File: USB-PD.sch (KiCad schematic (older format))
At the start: 54 parts, among them IC3 TPS7A0518PDBVT, J1 1053131102, J11 E8124-015-01, Q10 Si7223DN, Q11 Si7223DN, Q9 SQS401EN-T1_BE3, U12 STUSB4500QTR, U14 LTC4418IUF#PBF

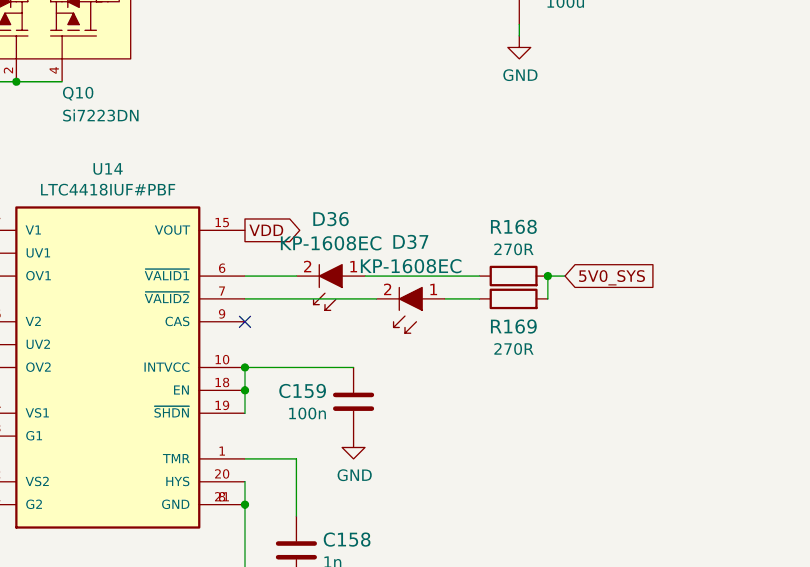
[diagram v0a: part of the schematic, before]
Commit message: All routes connected
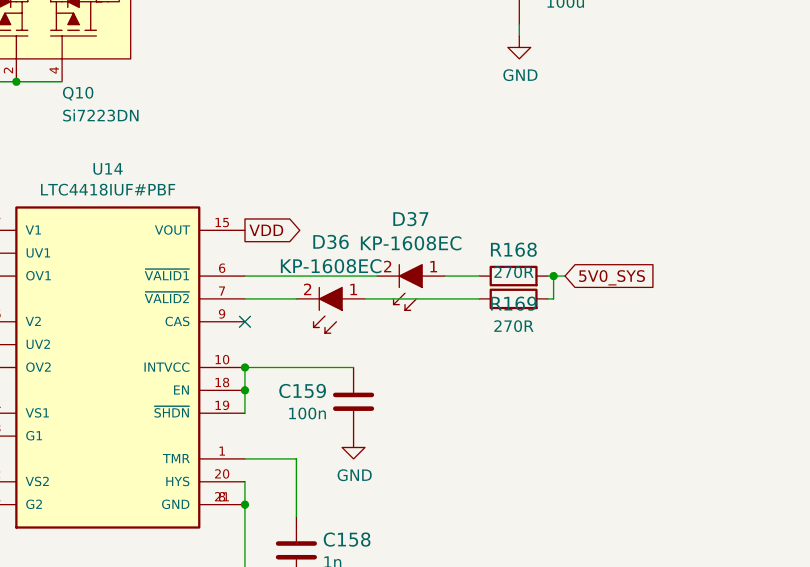
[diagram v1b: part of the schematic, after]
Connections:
- net at U14.6 (~VALID1): now also D37.2; no longer D36.2
- net at U14.7 (~VALID2): now also D36.2; no longer D37.2
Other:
- moved on the sheet: D36, D37, R168, R169
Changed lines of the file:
@@
 L sc606-baseboard:KP-1608EC D?
 U 1 1 62106E33
-P 9650 8200
+P 9650 8300
 AR Path="/61D43102/62106E33" Ref="D?"  Part="1"
 AR Path="/61D49FDE/62106E33" Ref="D?"  Part="1"
 AR Path="/623AED4D/62106E33" Ref="D36"  Part="1"
-F 0 "D36" H 9600 7953 60  0000 C CNN
-F 1 "KP-1608EC" H 9600 8059 60  0000 C CNN
-F 2 "sc606-baseboard-footprints:LED_0603" H 9850 8400 60  0001 L CNN
-F 3 "https://www.farnell.com/datasheets/1854072.pdf" H 9850 8500 60  0001 L CNN
-F 4 "KP-1608EC" H 9850 8700 60  0001 L CNN "MPN"
-F 5 "KINGBRIGHT" H 9860 8820 60  0001 L CNN "Manufacturer"
-	1    9650 8200
+F 0 "D36" H 9600 8053 60  0000 C CNN
+F 1 "KP-1608EC" H 9600 8159 60  0000 C CNN
+F 2 "sc606-baseboard-footprints:LED_0603" H 9850 8500 60  0001 L CNN
+F 3 "https://www.farnell.com/datasheets/1854072.pdf" H 9850 8600 60  0001 L CNN
+F 4 "KP-1608EC" H 9850 8800 60  0001 L CNN "MPN"
+F 5 "KINGBRIGHT" H 9860 8920 60  0001 L CNN "Manufacturer"
+	1    9650 8300
 	-1   0    0    1
 $EndComp
@@
 L sc606-baseboard:KP-1608EC D?
 U 1 1 6211676C
-P 10000 8300
+P 10000 8200
 AR Path="/61D43102/6211676C" Ref="D?"  Part="1"
 AR Path="/61D49FDE/6211676C" Ref="D?"  Part="1"
 AR Path="/623AED4D/6211676C" Ref="D37"  Part="1"
-F 0 "D37" H 9950 8053 60  0000 C CNN
-F 1 "KP-1608EC" H 9950 8159 60  0000 C CNN
-F 2 "sc606-baseboard-footprints:LED_0603" H 10200 8500 60  0001 L CNN
-F 3 "https://www.farnell.com/datasheets/1854072.pdf" H 10200 8600 60  0001 L CNN
-F 4 "KP-1608EC" H 10200 8800 60  0001 L CNN "MPN"
-F 5 "KINGBRIGHT" H 10210 8920 60  0001 L CNN "Manufacturer"
-	1    10000 8300
+F 0 "D37" H 9950 7953 60  0000 C CNN
+F 1 "KP-1608EC" H 9950 8059 60  0000 C CNN
+F 2 "sc606-baseboard-footprints:LED_0603" H 10200 8400 60  0001 L CNN
+F 3 "https://www.farnell.com/datasheets/1854072.pdf" H 10200 8500 60  0001 L CNN
+F 4 "KP-1608EC" H 10200 8700 60  0001 L CNN "MPN"
+F 5 "KINGBRIGHT" H 10210 8820 60  0001 L CNN "Manufacturer"
+	1    10000 8200
 	-1   0    0    1
 $EndComp
@@
 L sc606-baseboard:R_270R_0603 R168
 U 1 1 6201E54F
+P 10500 8300
+F 0 "R168" H 10500 8513 60  0000 C CNN
+F 1 "R_270R_0603" H 10500 8150 60  0001 C CNN
+F 2 "sc606-baseboard-footprints:0603-res" H 10700 8500 60  0001 L CNN
+F 3 "https://industrial.panasonic.com/cdbs/www-data/pdf/RDA0000/AOA0000C304.pdf" H 10500 8300 50  0001 C CNN
+F 4 "Panasonic" H 10700 8700 60  0001 L CNN "Manufacturer"
+F 5 "ERJ3EKF2700V" H 10700 8600 60  0001 L CNN "MPN"
+F 6 "270R" H 10500 8415 50  0000 C CNN "Val"
+	1    10500 8300
+	1    0    0    -1
+$EndComp
+$Comp
+L sc606-baseboard:R_270R_0603 R169
+U 1 1 6201EDA2
 P 10500 8200
-F 0 "R168" H 10500 8413 60  0000 C CNN
+F 0 "R169" H 10500 8077 60  0000 C CNN
 F 1 "R_270R_0603" H 10500 8050 60  0001 C CNN
 F 2 "sc606-baseboard-footprints:0603-res" H 10700 8400 60  0001 L CNN
@@
 F 4 "Panasonic" H 10700 8600 60  0001 L CNN "Manufacturer"
 F 5 "ERJ3EKF2700V" H 10700 8500 60  0001 L CNN "MPN"
-F 6 "270R" H 10500 8315 50  0000 C CNN "Val"
+F 6 "270R" H 10500 7979 50  0000 C CNN "Val"
 	1    10500 8200
 	1    0    0    -1
 $EndComp
-$Comp
-L sc606-baseboard:R_270R_0603 R169
-U 1 1 6201EDA2
-P 10500 8300
-F 0 "R169" H 10500 8177 60  0000 C CNN
-F 1 "R_270R_0603" H 10500 8150 60  0001 C CNN
-F 2 "sc606-baseboard-footprints:0603-res" H 10700 8500 60  0001 L CNN
-F 3 "https://industrial.panasonic.com/cdbs/www-data/pdf/RDA0000/AOA0000C304.pdf" H 10500 8300 50  0001 C CNN
-F 4 "Panasonic" H 10700 8700 60  0001 L CNN "Manufacturer"
-F 5 "ERJ3EKF2700V" H 10700 8600 60  0001 L CNN "MPN"
-F 6 "270R" H 10500 8079 50  0000 C CNN "Val"
-	1    10500 8300
-	1    0    0    -1
-$EndComp
-Wire Wire Line
-	10350 8200 9850 8200
-Wire Wire Line
-	10200 8300 10350 8300
-Wire Wire Line
-	9900 8300 9325 8300
-Wire Wire Line
-	9325 8200 9550 8200
+Wire Wire Line
+	10200 8200 10350 8200
 Text GLabel 10725 8200 2    50   Input ~ 0
 5V0_SYS
-Wire Wire Line
-	10650 8200 10650 8300
-Wire Wire Line
-	10725 8200 10650 8200
-Connection ~ 10650 8200
 Wire Wire Line
 	7800 9100 7800 9350
@@
 Text Notes 2350 950  0    50   ~ 0
 9...20 VDC
+Wire Wire Line
+	9550 8300 9325 8300
+Wire Wire Line
+	9850 8300 10350 8300
+Wire Wire Line
+	9325 8200 9900 8200
+Wire Wire Line
+	10650 8300 10675 8300
+Wire Wire Line
+	10675 8300 10675 8200
+Wire Wire Line
+	10650 8200 10675 8200
+Connection ~ 10675 8200
+Wire Wire Line
+	10675 8200 10725 8200
 $EndSCHEMATC
